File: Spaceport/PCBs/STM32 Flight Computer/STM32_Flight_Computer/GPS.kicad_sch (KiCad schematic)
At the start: 1 part, among them U4 SAM-M8Q

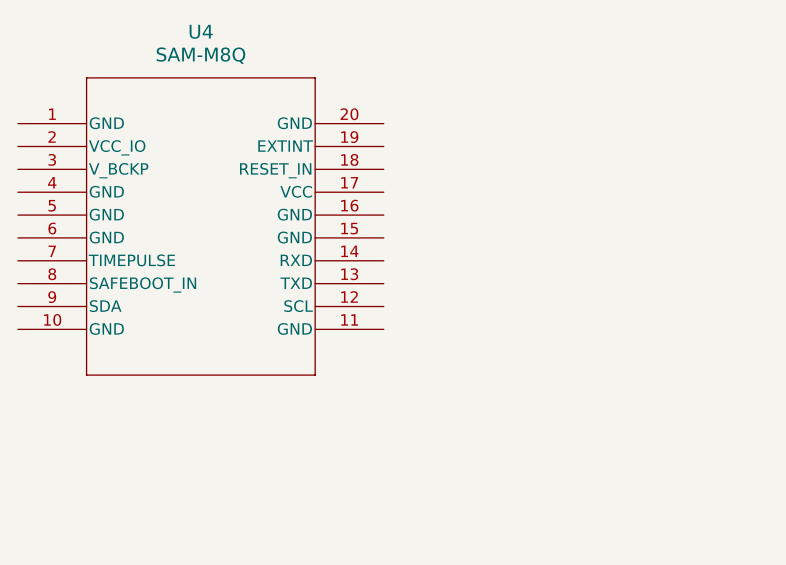
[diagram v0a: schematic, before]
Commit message: GPS Subcircuit
- Note: VCC_IO, VCC_BCKP and VCC are tied based on integration manual

- Integration manual https://github.com/xioTechnologies/SAM-M8Q-Breakout/blob/master/SAM-M8Q%20Datasheet.pdf
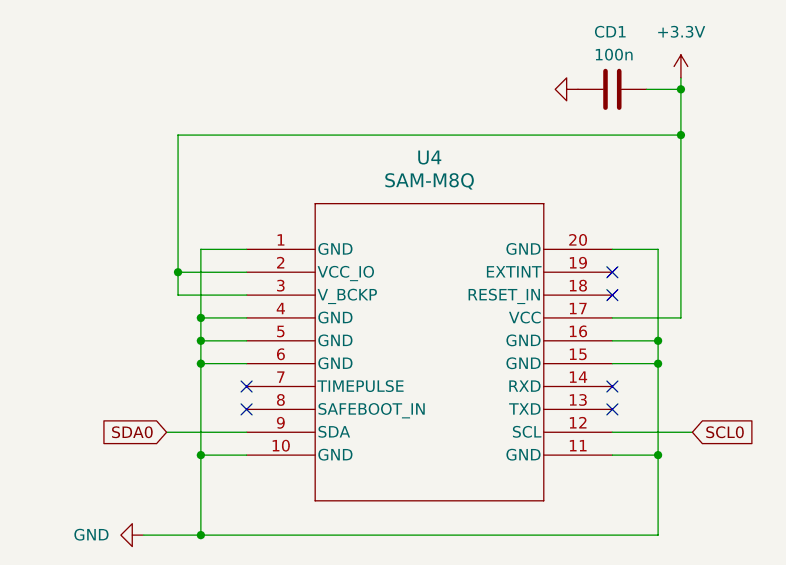
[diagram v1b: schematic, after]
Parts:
- added CD1: 100n, Capacitor_SMD:C_0603_1608Metric, symbol Device:C
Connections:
- net GND: now reaches U4.1 (GND)
- net GND: now also U4.10 (GND), U4.11 (GND), U4.15 (GND), U4.16 (GND), U4.20 (GND), U4.4 (GND), U4.5 (GND), U4.6 (GND), CD1.2
- net SCL0: now reaches U4.12 (SCL)
- net +3.3V: now reaches U4.17 (VCC)
- net +3.3V: now also U4.2 (VCC_IO), U4.3 (V_BCKP), CD1.1
- net SDA0: now reaches U4.9 (SDA)
- no-connect marks 0 -> 6
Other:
- moved on the sheet: U4
